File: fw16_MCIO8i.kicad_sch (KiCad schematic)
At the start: 31 parts

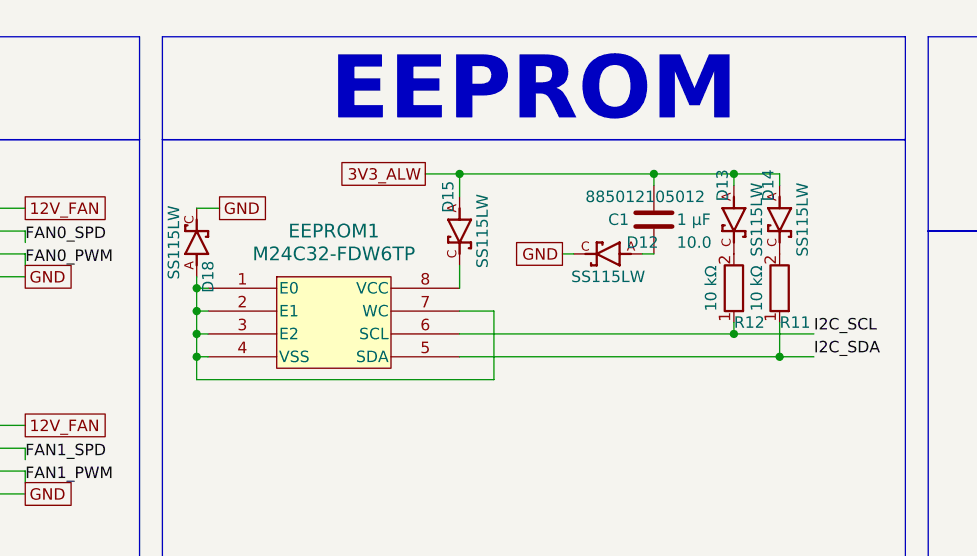
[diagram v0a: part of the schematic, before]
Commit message: README and cleanup
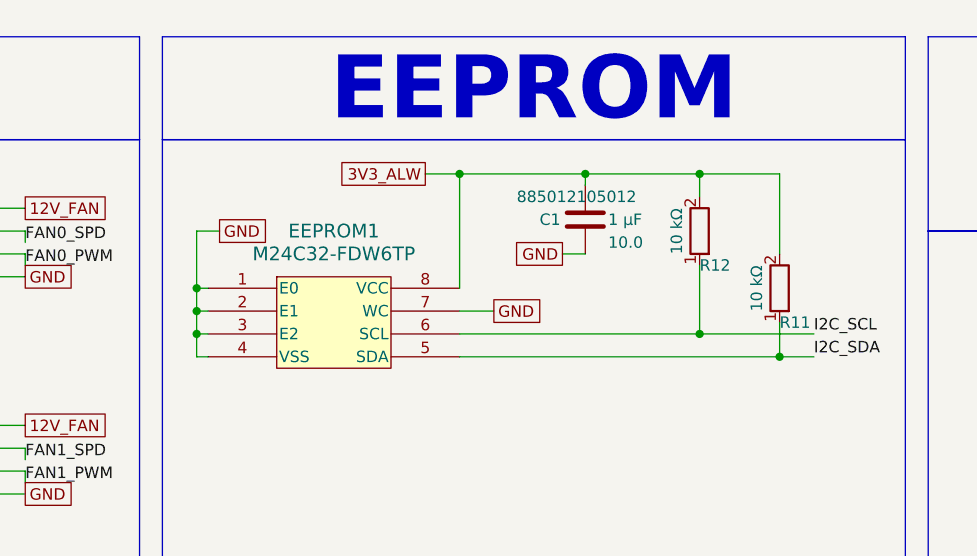
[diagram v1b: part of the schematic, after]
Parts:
- removed D12, D13, D14, D15, D18: SS115LW, diode:DIO_SS115LW, symbol diode:SS115LW
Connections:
- net 3V3_ALW: now also EEPROM1.8 (VCC), R11.2, R12.2
- net GND: now also C1.2, EEPROM1.1 (E0), EEPROM1.2 (E1), EEPROM1.3 (E2), EEPROM1.4 (VSS), EEPROM1.7 (WC)
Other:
- moved on the sheet: C1, R12
